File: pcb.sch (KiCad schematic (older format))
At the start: 5 parts, among them U1 STM32F103C8T6, U2 Shaft_encoder, U3 compass_accelerometer

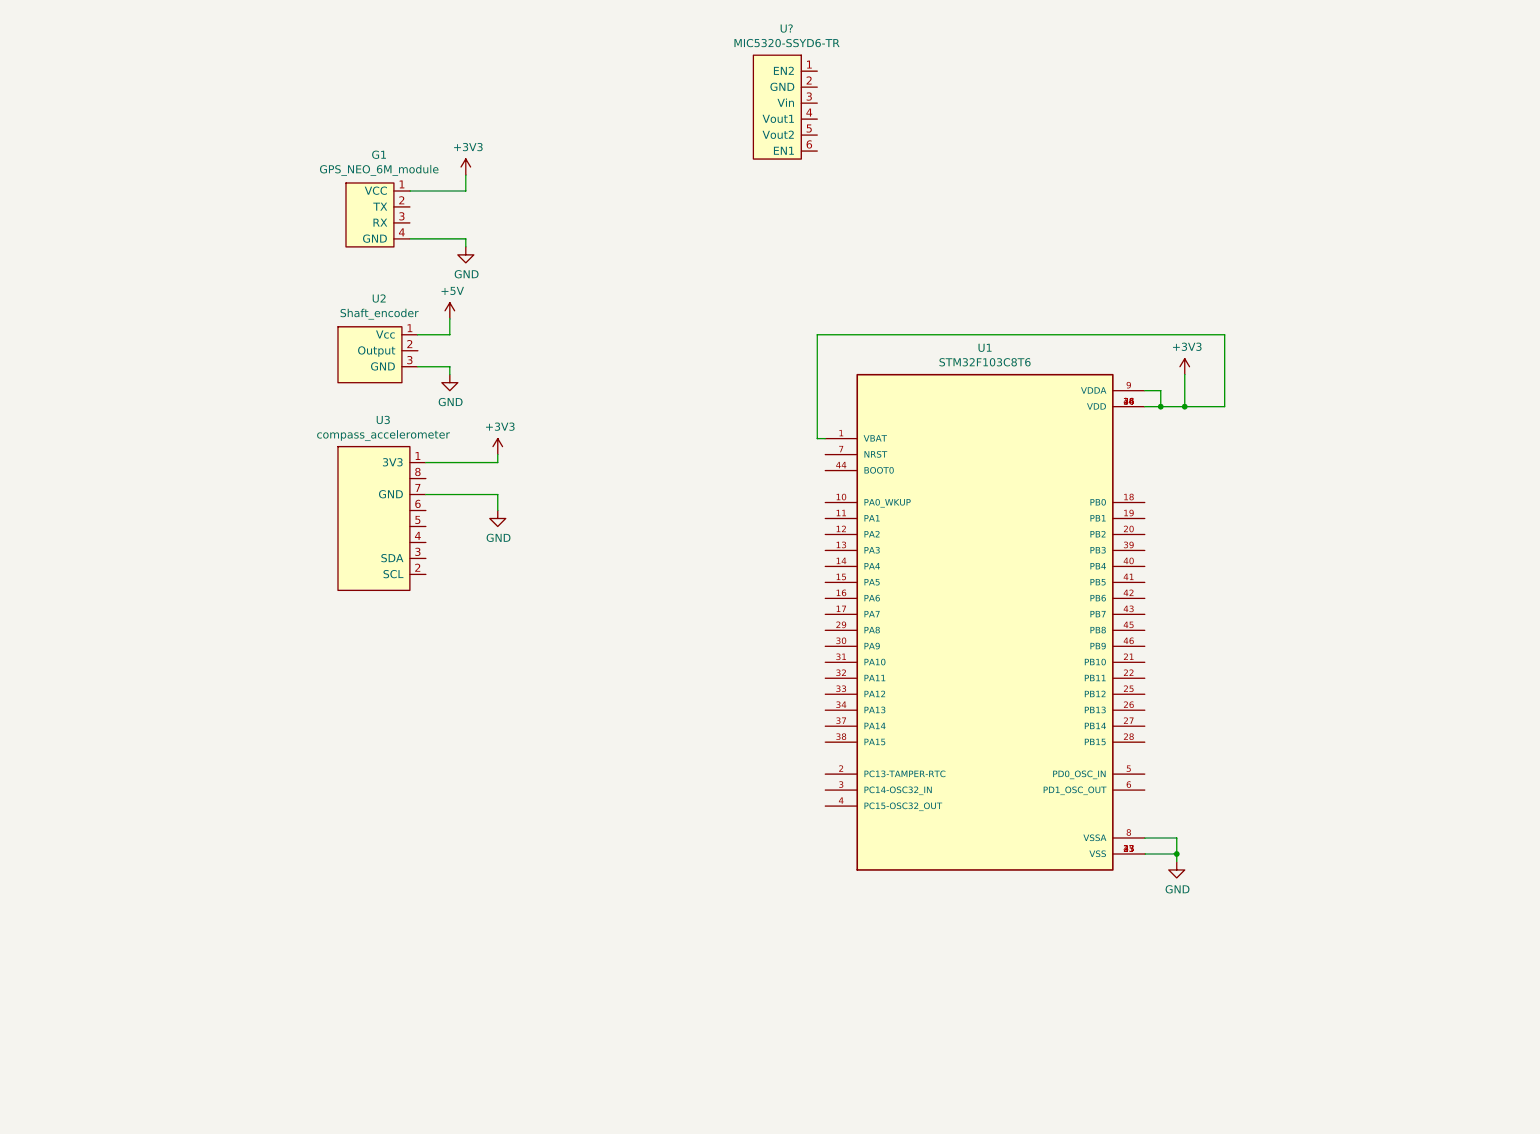
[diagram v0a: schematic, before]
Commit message: finished power supply
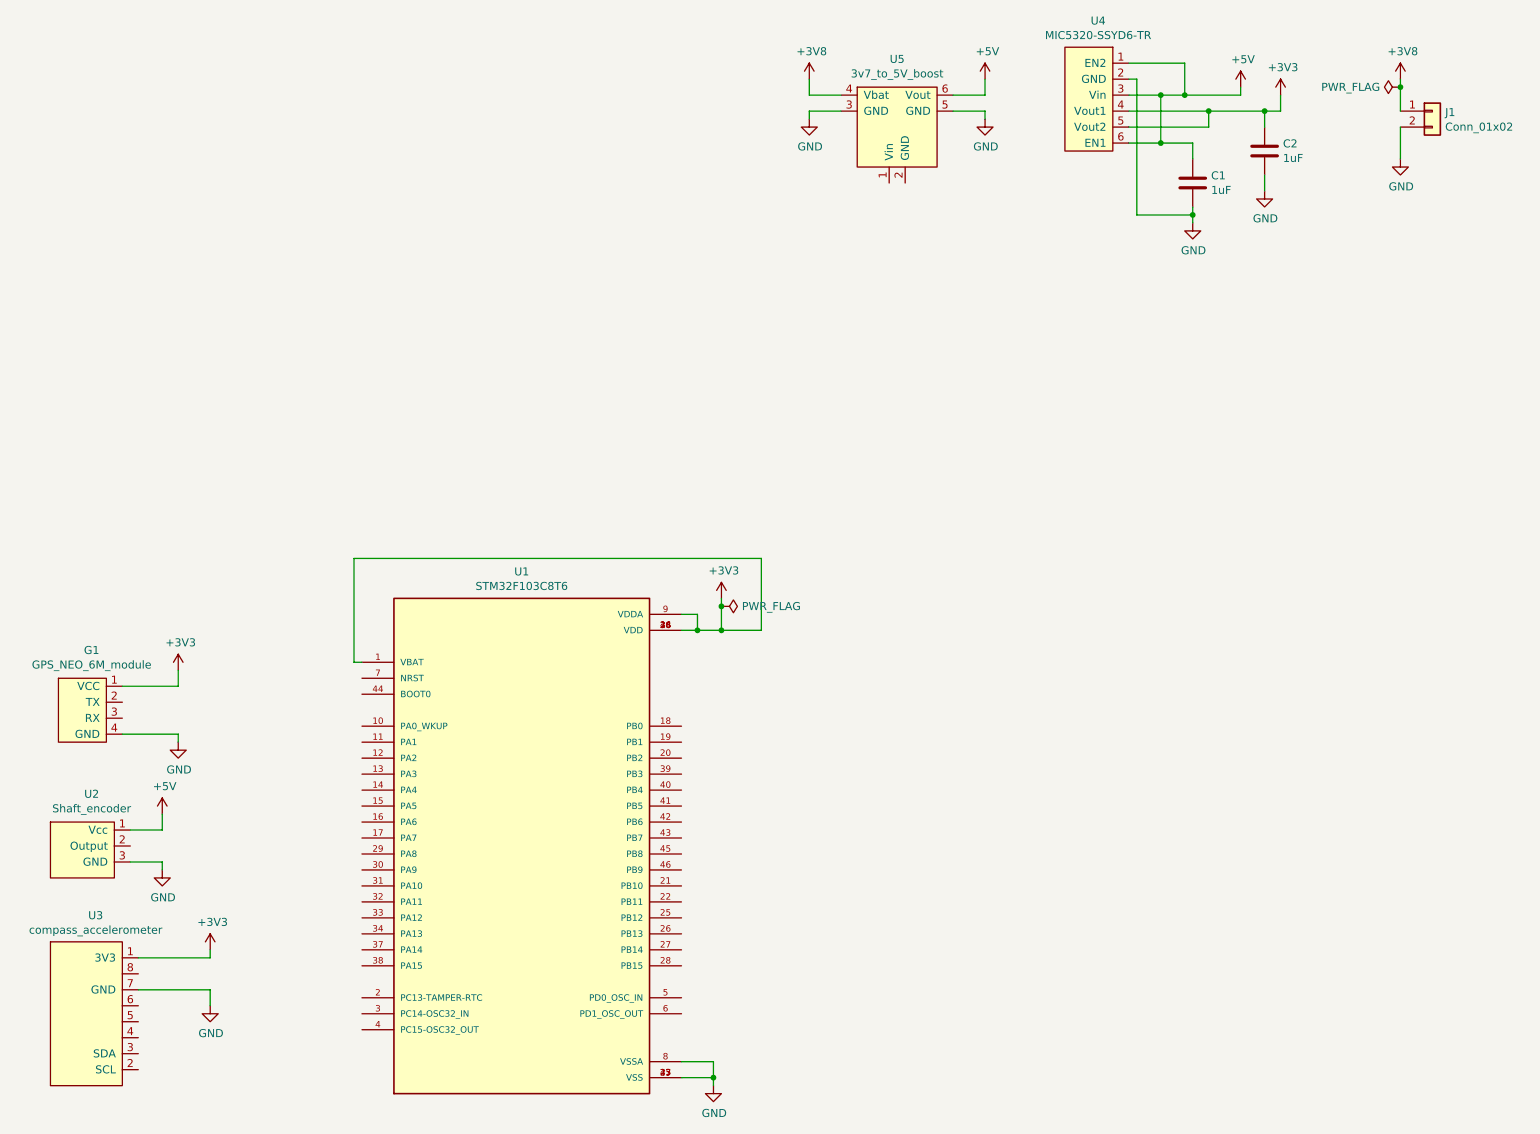
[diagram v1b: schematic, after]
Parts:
- added C1, C2: 1uF, symbol device:C
- added J1: Conn_01x02, symbol Connector_Generic:Conn_01x02
- added U5: 3v7_to_5V_boost, components_ece445:3v7_to_5V_boost, symbol components_senior_design:3v7_to_5V_boost
- gave numbers to parts that had none: 1
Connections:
- net +3V3: now also U4.4 (Vout1), U4.5 (Vout2), C2.1
- net +5V: now also U4.1 (EN2), U4.3 (Vin), U4.6 (EN1), C1.1, U5.6 (Vout)
- net GND: now also U4.2 (GND), C1.2, C2.2, J1.2 (Pin_2), U5.3 (GND), U5.5 (GND)
- new net +3V8: J1.1 (Pin_1), U5.4 (Vbat)
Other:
- moved on the sheet: G1, U1, U2, U3, U4
